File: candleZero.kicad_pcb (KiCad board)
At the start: 2 copper layers, 14 x 20.5 mm, 25 parts, among them J1 CONN_02X02, J5 CONN_02X05, J6 DB9_MALE, U1 STM32F072C8Ux, U2 TLV70233DBV, U3 TJA1051TK/3

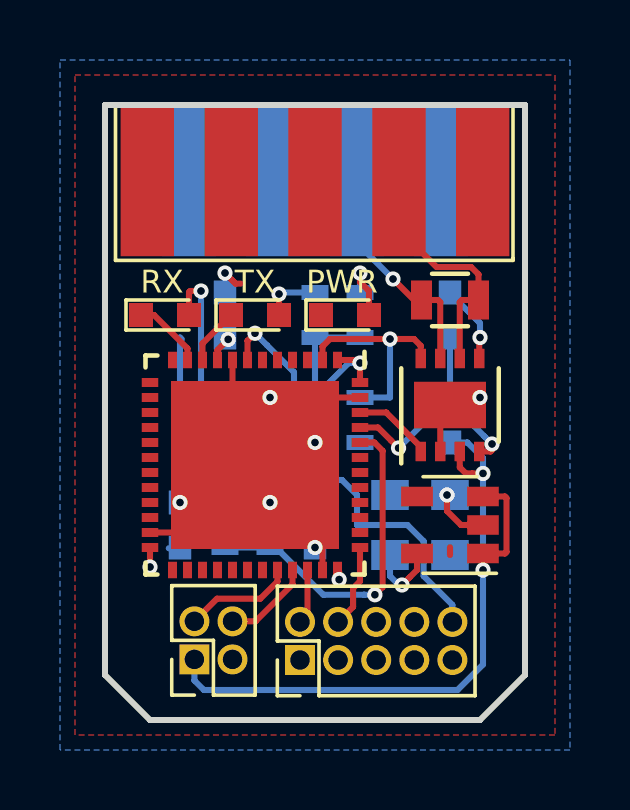
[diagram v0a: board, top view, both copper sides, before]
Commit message: v0.2
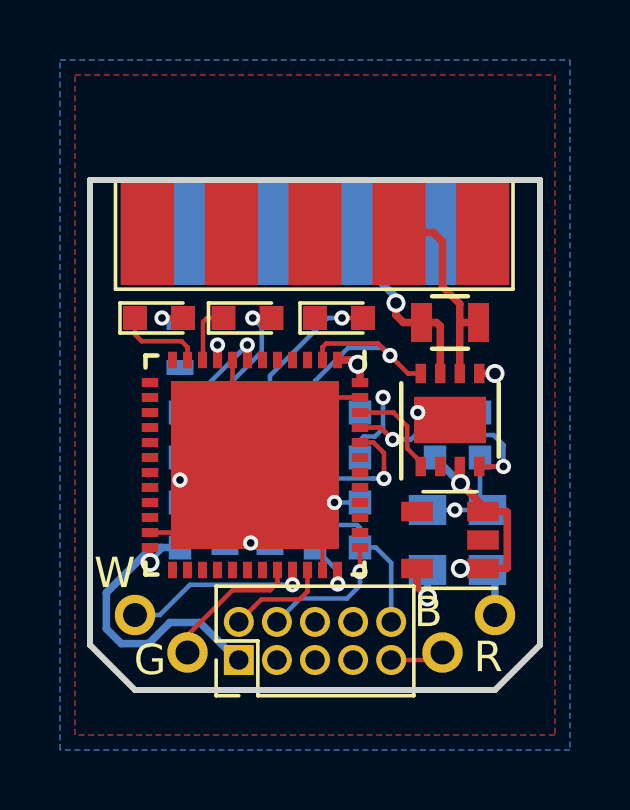
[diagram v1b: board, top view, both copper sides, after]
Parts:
- added J2: TEST_1P, pins:Pin_Header_Straight_1x01_Pitch2.00mm, F.Cu at (161.8, 101.2)
- added J3: TEST_1P, pins:Pin_Header_Straight_1x01_Pitch2.00mm, F.Cu at (153.2, 101.2)
- added J4: TEST_1P, pins:Pin_Header_Straight_1x01_Pitch2.00mm, F.Cu at (151.5, 100.0)
- J1: value CONN_02X02 -> TEST_1P; footprint Pin_Headers:Pin_Header_Straight_2x02_Pitch1.27mm -> pins:Pin_Header_Straight_1x01_Pitch2.00mm
- J6: footprint Connectors:DB9M_CI -> subd9-small:DB9M_CI_SMALL
- moved J1 10.1 mm to (163.5, 100.0), turned to 270 degrees
- moved R5 5.00 mm to (156.0, 94.0)
- moved R6 5.00 mm to (154.5, 94.0)
- moved C2 4.61 mm to (159.0, 97.0)
- moved C1 4.27 mm to (153.0, 94.0), turned to 270 degrees
- moved C5 4.12 mm to (163.0, 94.0)
- moved R7 2.92 mm to (153.0, 91.0), turned to 90 degrees
- moved J6 2.54 mm to (157.5, 88.0)
- moved J5 2.04 mm to (155.0, 101.5)
- moved C8 1.58 mm to (159.0, 94.0)
- moved R3 1.58 mm to (157.5, 94.0)
- moved C4 1.35 mm to (163.2, 97.5)
- moved C7 1.35 mm to (161.2, 97.5)
- moved R4 0.75 mm to (162.0, 90.2)
- moved C6 0.71 mm to (161.5, 94.0)
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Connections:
- net Net-(J6-Pad2) renamed /CAN_L
- net Net-(J6-Pad7) renamed /CAN_H
- J5 pad 7: Net-(J5-Pad7) -> GND
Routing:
- net +5V: track 25.7 -> 10.4 mm
- net GND: track 35.7 -> 27.9 mm, vias 8 -> 6
- net Net-(D3-Pad2): track 7.04 -> 1.35 mm
- net Net-(R1-Pad2): track 11.6 -> 7.68 mm
- net +3V3: track 14.5 -> 17.9 mm
- net USB_DP: track 2.99 -> 6.16 mm, vias 0 -> 1
- net Net-(D1-Pad2): track 2.22 -> 5.12 mm
- net Net-(D2-Pad2): track 1.92 -> 4.41 mm
- net (no net): track 2.34 -> 0.00 mm
- net SWCLK: track 2.78 -> 4.54 mm, vias 0 -> 1
- net SWDIO: track 1.83 -> 3.42 mm
- net /CAN_L: track 8.31 -> 9.39 mm
- net /CAN_H: track 7.57 -> 6.50 mm
- net USB_DM: track 3.70 -> 4.73 mm
- net CAN_S: track 7.60 -> 8.28 mm
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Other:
- board size 14 x 20.5 mm -> 15 x 17 mm
- net class 3V3 added: clearance 0.1524, trace_width 0.254, via_dia 0.635, via_drill 0.381
- net class 5V added: clearance 0.1524, trace_width 0.254, via_dia 0.635, via_drill 0.381
- net class CAN added: clearance 0.1524, trace_width 0.254, via_dia 0.635, via_drill 0.381
- net class Default: trace_width 0.2032 -> 0.1524
- rule trace_min: 0.127 -> 0.1524
- board text added: "candleZero bytewerk.org"
- board text added: "v0.2"
- board text removed: "PWR"
- board text removed: "RX"
- board text removed: "TX"
- board text removed: "candleZero v0.1"
- board text removed: "https://bytewerk.org/"

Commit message: v0.3
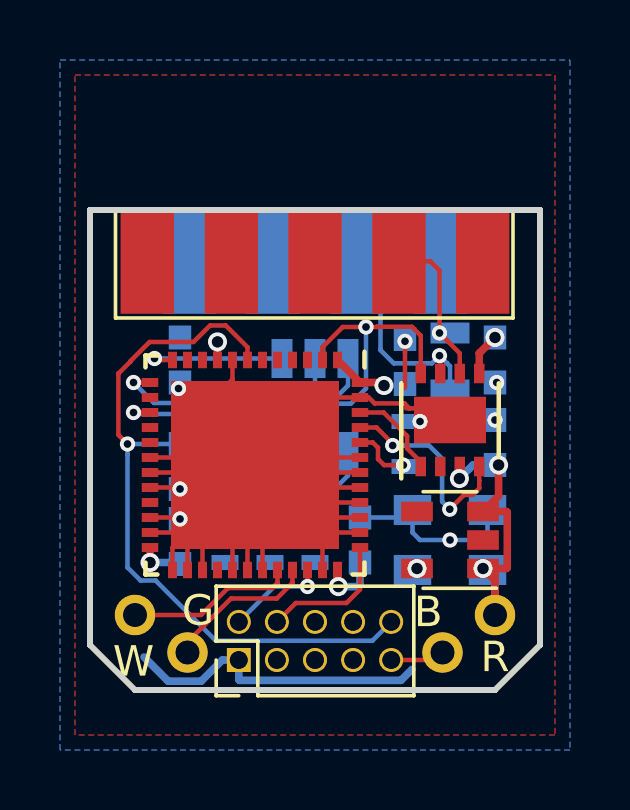
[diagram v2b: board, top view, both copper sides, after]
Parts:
- removed D2, D3: LED, LEDs:LED_0603
- removed R1: dnp, Resistors_SMD:R_0603
- D1: value LED -> LED_RGB; footprint LEDs:LED_0603 -> LEDs:LED_RGB_PLCC-6; moved to B.Cu
- J5: footprint Pin_Headers:Pin_Header_Straight_2x05_Pitch1.27mm -> jtag:Pin_Header_Straight_2x05_Pitch1.27mm
- R4: moved to B.Cu
- moved C9 9.27 mm to (160.5, 91.5)
- moved R7 7.91 mm to (157.5, 97.5)
- moved C2 6.31 mm to (153.0, 95.0), turned to 270 degrees
- moved R2 5.25 mm to (160.5, 94.3), turned to 90 degrees
- moved C3 4.53 mm to (153.0, 97.5)
- moved R5 3.81 mm to (154.5, 97.5)
- moved R6 3.81 mm to (156.0, 97.5)
- moved C8 3.50 mm to (159.0, 97.5), turned to 90 degrees
- moved R3 3.18 mm to (154.5, 95.0)
- moved D1 3.01 mm to (157.5, 93.0), turned to 270 degrees
- moved C5 2.55 mm to (163.5, 91.5)
- moved C1 2.50 mm to (153.0, 91.5)
- moved J3 2.15 mm to (151.5, 100.0)
- moved J4 2.15 mm to (153.2, 101.2)
- moved C6 2.02 mm to (163.5, 94.2)
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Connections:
- net Net-(R1-Pad2) renamed /BOOT
- D1 pad 1: GND -> LED_R
- D1 pad 2: Net-(D1-Pad2) -> LED_G
- R5 pad 2: Net-(D1-Pad2) -> Net-(D1-Pad6)
- R6 pad 2: Net-(D2-Pad2) -> Net-(D1-Pad5)
- R7 pad 2: Net-(D3-Pad2) -> Net-(D1-Pad4)
- U1 pad 10: LED1 -> Net-(U1-Pad10)
- U1 pad 11: LED2 -> Net-(U1-Pad11)
- U1 pad 12: Net-(U1-Pad12) -> LED_R
- U1 pad 13: Net-(U1-Pad13) -> LED_G
- U1 pad 15: Net-(U1-Pad15) -> LED_B
- U1 pad 18: Net-(U1-Pad18) -> GND
- U1 pad 19: Net-(U1-Pad19) -> GND
- U1 pad 20: Net-(U1-Pad20) -> GND
- U1 pad 21: Net-(U1-Pad21) -> GND
- U1 pad 22: Net-(U1-Pad22) -> GND
- U1 pad 25: Net-(U1-Pad25) -> GND
- U1 pad 26: Net-(U1-Pad26) -> GND
- U1 pad 27: Net-(U1-Pad27) -> GND
- U1 pad 28: Net-(U1-Pad28) -> GND
- U1 pad 29: Net-(U1-Pad29) -> GND
- U1 pad 30: Net-(U1-Pad30) -> GND
- U1 pad 31: Net-(U1-Pad31) -> GND
- U1 pad 38: Net-(U1-Pad38) -> GND
- U1 pad 39: Net-(U1-Pad39) -> GND
- U1 pad 40: Net-(U1-Pad40) -> GND
- U1 pad 41: Net-(U1-Pad41) -> GND
- U1 pad 42: Net-(U1-Pad42) -> GND
- U1 pad 43: Net-(U1-Pad43) -> GND
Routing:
- net GND: track 27.9 -> 66.1 mm, vias 6 -> 8
- net LED_B: track 0.00 -> 9.01 mm, vias 0 -> 1
- net NRST: track 16.1 -> 24.1 mm
- net LED_G: track 0.00 -> 7.97 mm, vias 0 -> 1
- net /BOOT: track 7.68 -> 1.98 mm
- net CAN_S: track 8.28 -> 13.4 mm
- net Net-(D1-Pad2): track 5.12 -> 0.00 mm, vias 1 -> 0
- net LED_R: track 0.00 -> 4.87 mm, vias 0 -> 1
- net Net-(D2-Pad2): track 4.41 -> 0.00 mm, vias 1 -> 0
- net Net-(D1-Pad6): track 0.00 -> 3.55 mm
- net Net-(D1-Pad5): track 0.00 -> 3.42 mm
- net /CAN_L: track 9.39 -> 6.18 mm, vias 0 -> 1
- net LED2: track 2.90 -> 0.00 mm
- net Net-(D1-Pad4): track 0.00 -> 2.66 mm
- net /CAN_H: track 6.50 -> 8.52 mm
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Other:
- board size 15 x 17 mm -> 15 x 16 mm
- net class CAN: trace_width 0.254 -> 0.1524; via_dia 0.635 -> 0.508; via_drill 0.381 -> 0.254
- board text added: "bytewerk.org"
- board text added: "candleZero"
- board text added: "v0.3"
- board text removed: "candleZero bytewerk.org"
- board text removed: "v0.2"

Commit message: v0.4
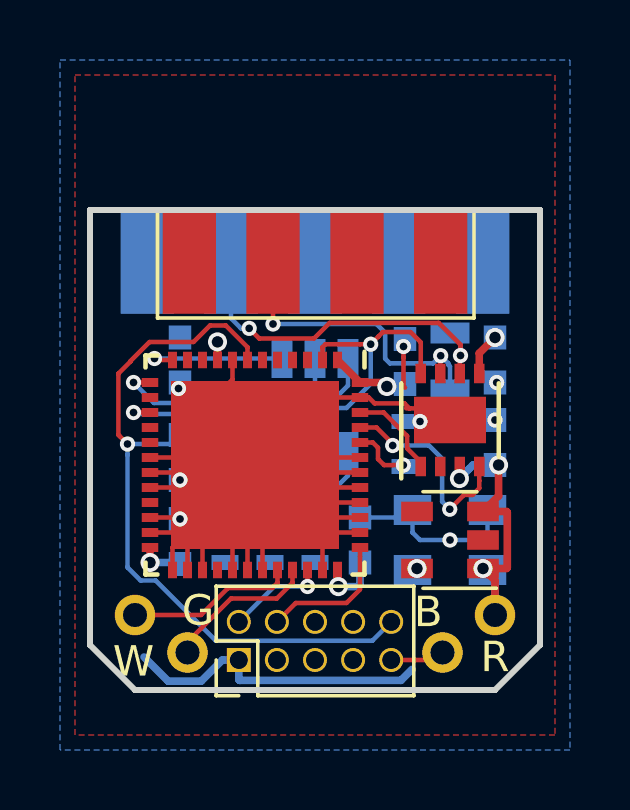
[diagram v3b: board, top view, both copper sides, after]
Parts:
- J6: moved to B.Cu
- moved C2 0.30 mm to (153.0, 94.8)
- moved R3 0.30 mm to (154.5, 94.8)
- turned J6 to 180 degrees
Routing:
- net /CAN_L: track 6.18 -> 12.2 mm, vias 1 -> 2
- net /CAN_H: track 8.52 -> 10.7 mm, vias 1 -> 2
- net CAN_S: track 13.4 -> 12.3 mm
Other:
- board text added: "v0.4"
- board text removed: "v0.3"
